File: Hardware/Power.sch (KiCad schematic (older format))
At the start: 23 parts, among them Q201 2N7000, U201 TPS63002DRCR, U202 TPS63031DSKR

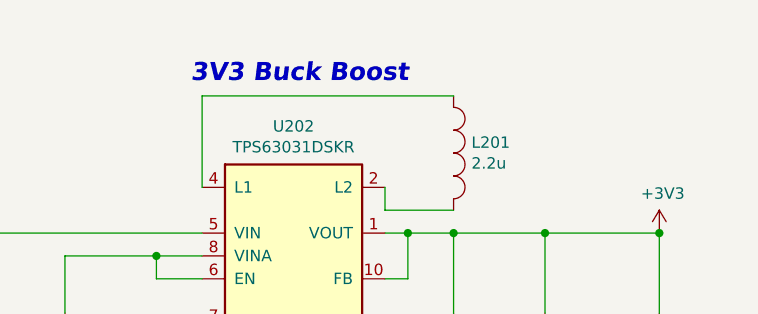
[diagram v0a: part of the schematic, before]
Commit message: save work at arges, finished layout and routing
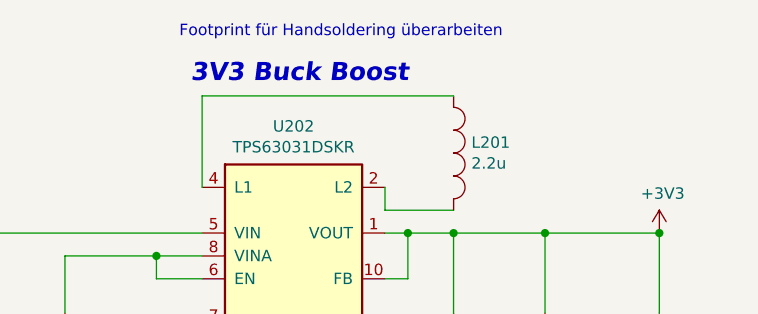
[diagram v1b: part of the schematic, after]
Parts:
- Q201: footprint digikey-footprints:TO-92-3 -> Digikey:TO-92-3
- TP201, TP202: footprint digikey-footprints:Test_Point_D1.02mm -> Digikey:Test_Point_D1.02mm
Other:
- note added: "Footprint für Handsoldering überarbeiten"

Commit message: savecommit
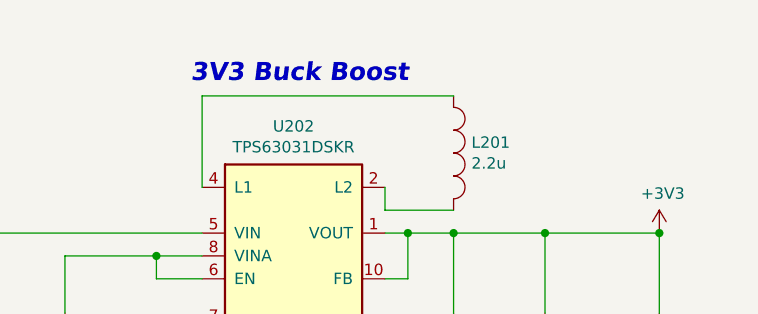
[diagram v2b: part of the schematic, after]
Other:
- note removed: "Footprint für Handsoldering überarbeiten"
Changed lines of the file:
@@
 EESchema Schematic File Version 4
-LIBS:E-Ink-cache
 EELAYER 30 0
 EELAYER END
@@
 Wire Wire Line
 	6400 4750 6900 4750
-Text Notes 7250 1000 0    50   ~ 0
-Footprint für Handsoldering überarbeiten
 Wire Wire Line
 	8450 1250 7350 1250
